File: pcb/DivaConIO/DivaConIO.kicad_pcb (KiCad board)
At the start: 2 copper layers, 65 x 75 mm, 74 parts, among them J1 B6B-PH-SM4-TBT, J2 B4B-PH-SM4-TBT, J3 B6B-PH-SM4-TBT, J4 Conn_01x05_MountingPin, J5 BM03B-SRSS-TBT, J6 B8B-PH-SM4-TBT, J7 B6B-PH-SM4-TBT, Q1 BSS138, Q2 BSS138, Q3 BSS138, Q4 BSS138, SW1 SW_Push, U1 74HCT1G14

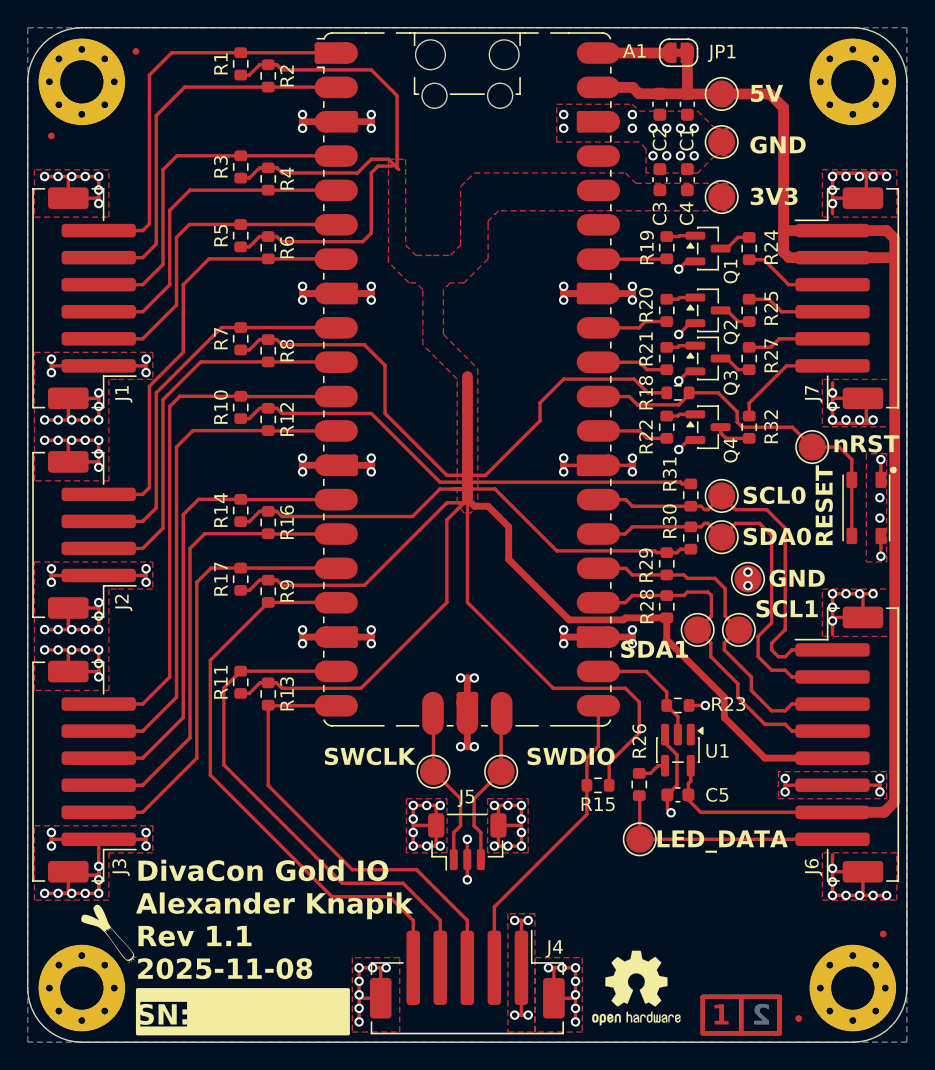
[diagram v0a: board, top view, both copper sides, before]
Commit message: generate revision 1.1 gerber files
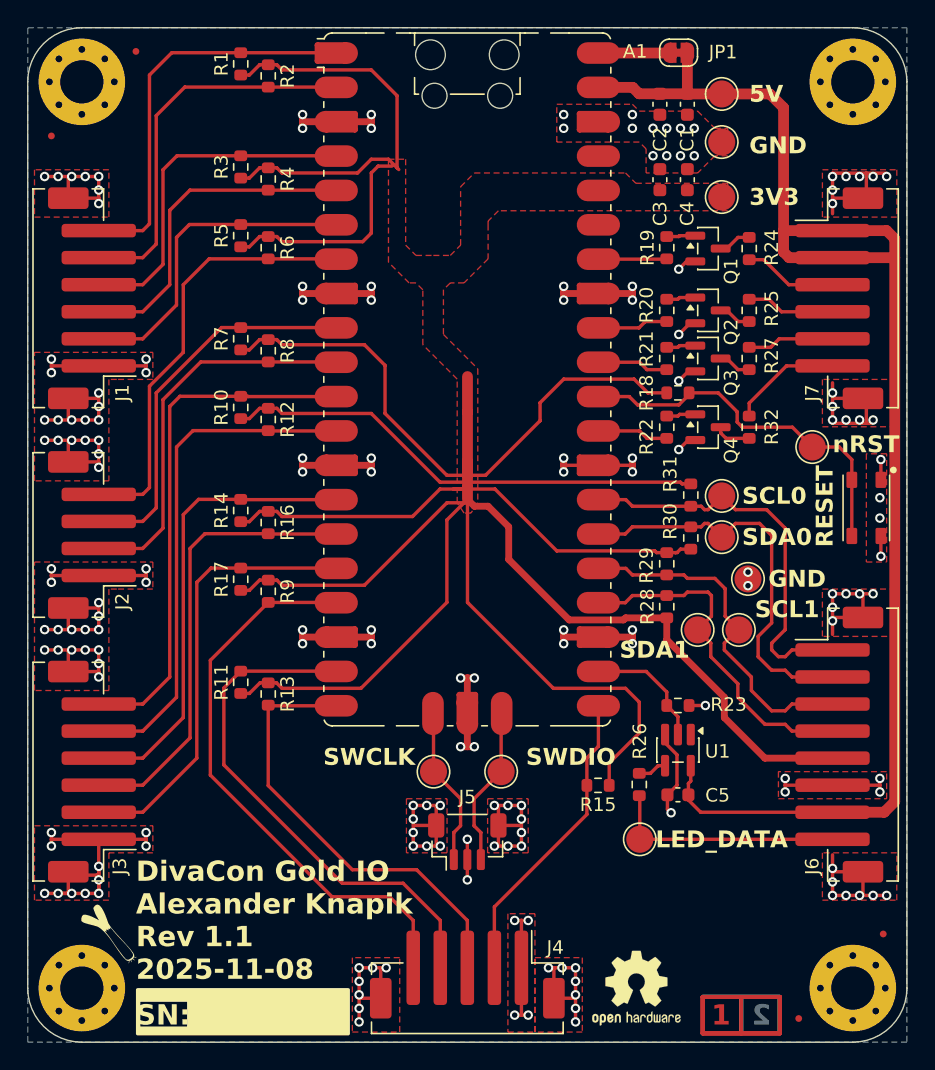
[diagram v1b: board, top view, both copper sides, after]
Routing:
- net GND: track 270.6 -> 270.0 mm
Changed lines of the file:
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@@
 	(segment
 		(start 124.892 116.218)
-		(end 128.956 112.154)
+		(end 130.988 110.122)
 		(width 0.254)
 		(layer "F.Cu")
@@
 	)
 	(segment
-		(start 130.988 110.122)
-		(end 128.956 112.154)
-		(width 0.254)
-		(layer "F.Cu")
-		(net 2)
-	)
-	(segment
 		(start 135.56 114.313032)
 		(end 135.56 111.9)
@@
 	)
 	(segment
-		(start 164.099 92)
-		(end 164.099 130)
-		(width 0.8)
-		(layer "F.Cu")
-		(net 4)
-	)
-	(segment
 		(start 155.88 90)
 		(end 155.88 91.58)
@@
 	)
 	(segment
-		(start 164.099 130)
+		(start 164.099 92)
 		(end 164.099 132.22)
 		(width 0.8)
@@
 	)
 	(segment
-		(start 147.119 127.26)
-		(end 147.119 127.869)
-		(width 0.254)
-		(layer "F.Cu")
-		(net 32)
-	)
-	(segment
 		(start 144.704 94.12)
 		(end 144.704 94.628)
@@
 		(width 0.254)
 		(layer "F.Cu")
-		(net 49)
-	)
-	(segment
-		(start 145.25 131.813)
-		(end 145.212 131.775)
-		(width 0.254)
-		(layer "F.Cu")
